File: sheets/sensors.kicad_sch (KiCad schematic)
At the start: 13 parts, among them CN1 StemmaQT, U2 BMP581, U3 SparkfunM9N, U5 ADXL375BCCZ-RL7, U7 ADXL345BCCZ-RL7

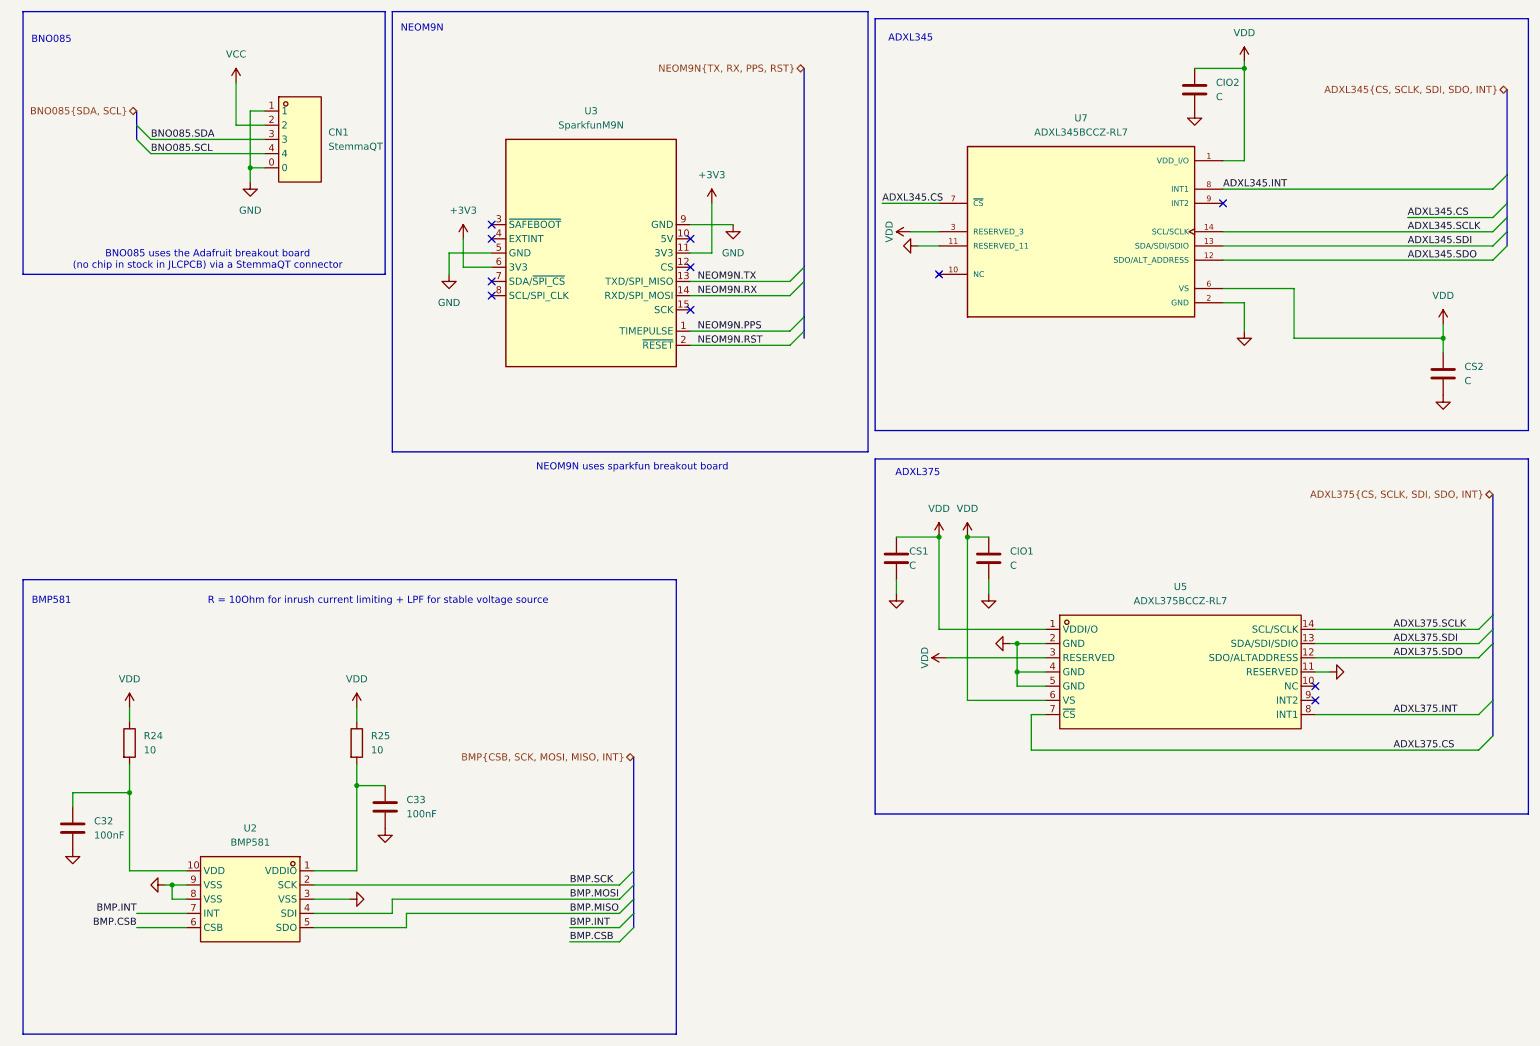
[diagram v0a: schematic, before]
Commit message: second push
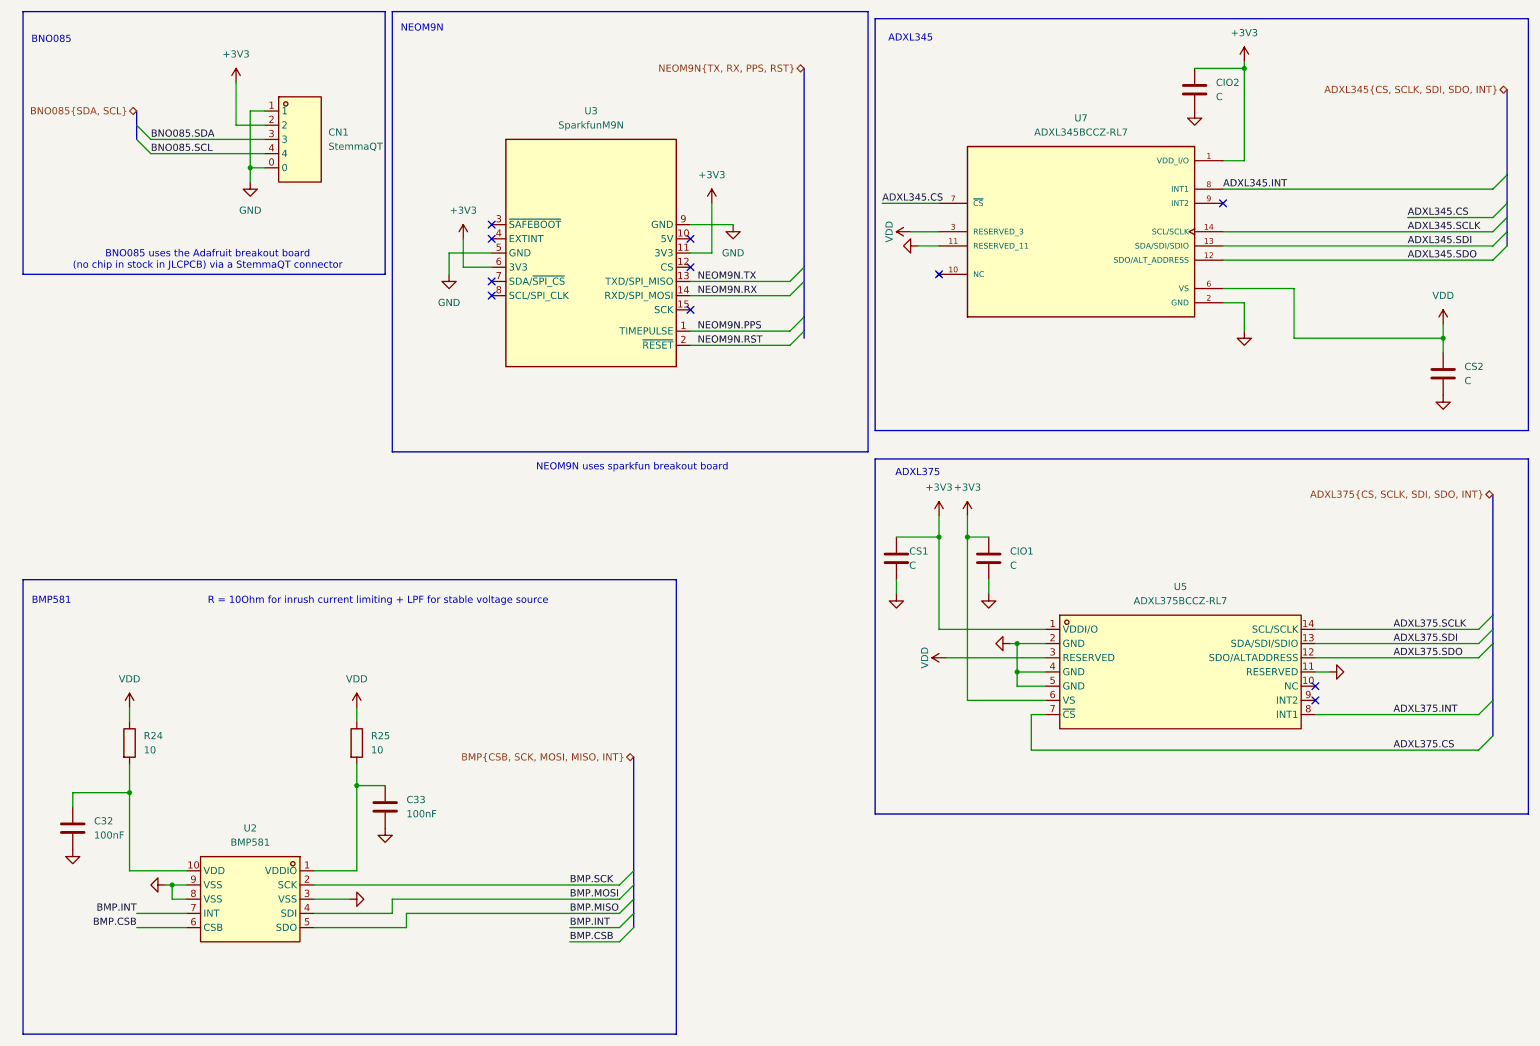
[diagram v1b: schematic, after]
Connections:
- net VCC is gone; now on net +3V3: CN1.2
- net +3V3: now also CIO1.1, CIO2.1, CS1.1, U5.1 (VDDI/O), U5.6 (VS), U7.1 (VDD_I/O)
- net VDD: no longer CIO1.1, CIO2.1, CS1.1, U5.1 (VDDI/O), U5.6 (VS), U7.1 (VDD_I/O)
